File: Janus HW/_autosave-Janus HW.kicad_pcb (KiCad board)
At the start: 4 copper layers, 38 x 20 mm, 22 parts, among them IC2 UM980, IC3 MP2338GTL-P, J1 USB_B_Micro, J2 Conn_Coaxial_Small, U1 ESP32-C3-MINI-1U-N4, U2 RFM69HCW

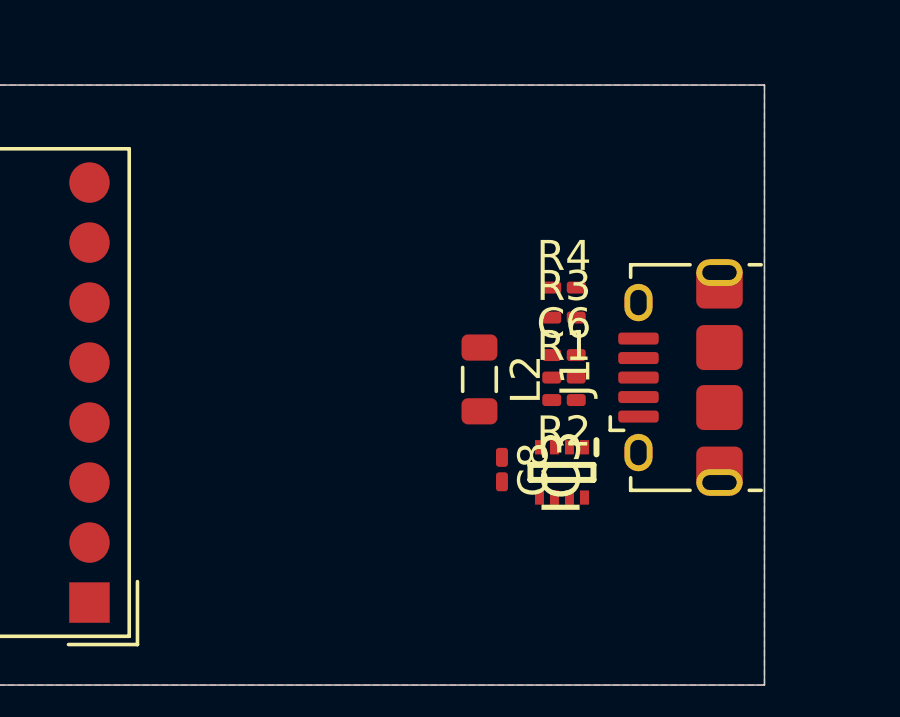
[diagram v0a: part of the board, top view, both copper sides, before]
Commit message: Fiddling in Kicad
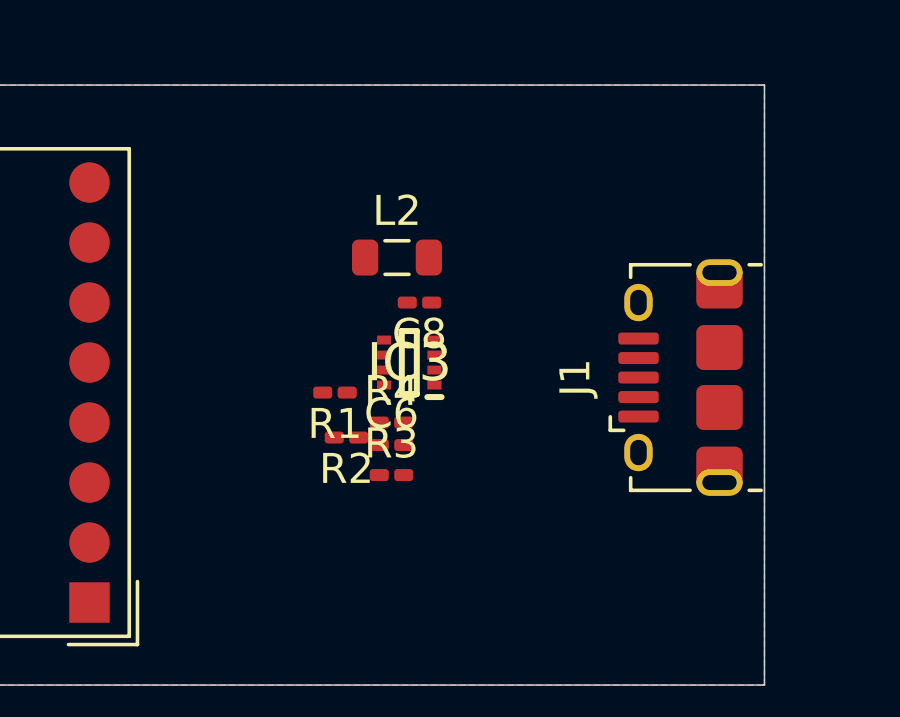
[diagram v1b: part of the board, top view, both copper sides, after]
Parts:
- moved R3 7.79 mm to (191.8, 69.0)
- moved R1 7.65 mm to (189.9, 66.2), turned to 180 degrees
- moved R2 7.36 mm to (190.3, 67.8)
- moved R4 7.30 mm to (191.8, 67.2)
- moved C6 6.49 mm to (191.8, 68.0)
- moved IC3 6.27 mm to (192.4, 65.2), turned to 180 degrees
- moved C8 6.21 mm to (192.8, 63.2), turned to 180 degrees
- moved L2 4.91 mm to (192.0, 61.8), turned to 0 degrees
